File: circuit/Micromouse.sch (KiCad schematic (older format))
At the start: 34 parts, among them J1 DBG_CN, J2 ICM-20602_1-4pin, J3 TEST_1P, J4 ICM-20602_5-8pin, J5 TEST_1P, J6 Conn_01x04, Q2 IRLML6344, SW2 SW_Push, SW3 SW_Push, SW4 SW_Push, U3 STM32F405RGTx

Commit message: Kicadのpcbnew映らないくてキレそう
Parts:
- D2, D3, D4, D5: footprint (none) -> LEDs:LED_0603
- J1: footprint (none) -> Socket_Strips:Socket_Strip_Straight_1x03_Pitch2.54mm
- J2, J4, J6: footprint (none) -> Socket_Strips:Socket_Strip_Straight_1x04_Pitch2.54mm
- R10, R5, R6, R9: footprint (none) -> Resistors_SMD:R_0603
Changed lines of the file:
@@
 F 0 "J4" H 5750 8650 50  0000 C CNN
 F 1 "ICM-20602_5-8pin" V 5850 8850 50  0000 C CNN
-F 2 "" H 5750 8950 50  0001 C CNN
+F 2 "Socket_Strips:Socket_Strip_Straight_1x04_Pitch2.54mm" H 5750 8950 50  0001 C CNN
 F 3 "~" H 5750 8950 50  0001 C CNN
 	1    5750 8950
@@
 F 0 "J6" H 12530 1742 50  0000 L CNN
 F 1 "Conn_01x04" H 12530 1651 50  0000 L CNN
-F 2 "" H 12450 1750 50  0001 C CNN
+F 2 "Socket_Strips:Socket_Strip_Straight_1x04_Pitch2.54mm" H 12450 1750 50  0001 C CNN
 F 3 "~" H 12450 1750 50  0001 C CNN
 	1    12450 1750
@@
 F 0 "R10" H 3670 10146 50  0000 L CNN
 F 1 "10k" H 3670 10055 50  0000 L CNN
-F 2 "" V 3530 10100 50  0001 C CNN
+F 2 "Resistors_SMD:R_0603" V 3530 10100 50  0001 C CNN
 F 3 "" H 3600 10100 50  0001 C CNN
 	1    3600 10100
@@
 F 0 "D5" V 3639 9532 50  0000 R CNN
 F 1 "DBG_LED2" V 3548 9532 50  0000 R CNN
-F 2 "" H 3600 9650 50  0001 C CNN
+F 2 "LEDs:LED_0603" H 3600 9650 50  0001 C CNN
 F 3 "" H 3600 9650 50  0001 C CNN
 	1    3600 9650
@@
 F 0 "J1" H 4618 9525 50  0000 C CNN
 F 1 "DBG_CN" H 4618 9616 50  0000 C CNN
-F 2 "" H 4700 9850 50  0001 C CNN
+F 2 "Socket_Strips:Socket_Strip_Straight_1x03_Pitch2.54mm" H 4700 9850 50  0001 C CNN
 F 3 "~" H 4700 9850 50  0001 C CNN
 	1    4700 9850
@@
 F 0 "R9" H 2970 10146 50  0000 L CNN
 F 1 "10k" H 2970 10055 50  0000 L CNN
-F 2 "" V 2830 10100 50  0001 C CNN
+F 2 "Resistors_SMD:R_0603" V 2830 10100 50  0001 C CNN
 F 3 "" H 2900 10100 50  0001 C CNN
 	1    2900 10100
@@
 F 0 "R6" H 2220 10146 50  0000 L CNN
 F 1 "10k" H 2220 10055 50  0000 L CNN
-F 2 "" V 2080 10100 50  0001 C CNN
+F 2 "Resistors_SMD:R_0603" V 2080 10100 50  0001 C CNN
 F 3 "" H 2150 10100 50  0001 C CNN
 	1    2150 10100
@@
 F 0 "R5" H 1470 10146 50  0000 L CNN
 F 1 "10k" H 1470 10055 50  0000 L CNN
-F 2 "" V 1330 10100 50  0001 C CNN
+F 2 "Resistors_SMD:R_0603" V 1330 10100 50  0001 C CNN
 F 3 "" H 1400 10100 50  0001 C CNN
 	1    1400 10100
@@
 F 0 "D4" V 2939 9532 50  0000 R CNN
 F 1 "DBG_LED1" V 2848 9532 50  0000 R CNN
-F 2 "" H 2900 9650 50  0001 C CNN
+F 2 "LEDs:LED_0603" H 2900 9650 50  0001 C CNN
 F 3 "" H 2900 9650 50  0001 C CNN
 	1    2900 9650
@@
 F 0 "D3" V 2189 9532 50  0000 R CNN
 F 1 "DBG_LED0" V 2098 9532 50  0000 R CNN
-F 2 "" H 2150 9650 50  0001 C CNN
+F 2 "LEDs:LED_0603" H 2150 9650 50  0001 C CNN
 F 3 "" H 2150 9650 50  0001 C CNN
 	1    2150 9650
@@
 F 0 "D2" V 1439 9533 50  0000 R CNN
 F 1 "TICK_LED" V 1348 9533 50  0000 R CNN
-F 2 "" H 1400 9650 50  0001 C CNN
+F 2 "LEDs:LED_0603" H 1400 9650 50  0001 C CNN
 F 3 "" H 1400 9650 50  0001 C CNN
 	1    1400 9650
@@
 F 0 "J2" H 5200 9050 50  0000 C CNN
 F 1 "ICM-20602_1-4pin" V 5300 8850 50  0000 C CNN
-F 2 "" H 5200 8850 50  0001 C CNN
+F 2 "Socket_Strips:Socket_Strip_Straight_1x04_Pitch2.54mm" H 5200 8850 50  0001 C CNN
 F 3 "~" H 5200 8850 50  0001 C CNN
 	1    5200 8850

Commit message: スーパーエンジニアの登竜門たる文彦は当然スーパーエンジニア
あってぃ許さない
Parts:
- C10, C11, C12, C13, C14, C15, C23, C5, C6, C7, C8, C9: footprint Capacitors_SMD:C_0603 -> Capacitor_SMD:C_0603_1608Metric
- D2, D3, D4, D5: footprint LEDs:LED_0603 -> LED_SMD:LED_0603_1608Metric
- J1: footprint Socket_Strips:Socket_Strip_Straight_1x03_Pitch2.54mm -> Connector_PinSocket_2.54mm:PinSocket_1x03_P2.54mm_Vertical
- J2, J4, J6: footprint Socket_Strips:Socket_Strip_Straight_1x04_Pitch2.54mm -> Connector_PinSocket_2.54mm:PinSocket_1x04_P2.54mm_Vertical
- J3, J5: footprint Measurement_Points:Measurement_Point_Round-SMD-Pad_Small -> TestPoint:TestPoint_Pad_D1.0mm
- LS1: symbol Audio:CSS-0575A-SMT -> Micromouse-rescue:CSS-0575A-SMT-Audio
- Q2: footprint TO_SOT_Packages_SMD:SOT-23 -> Package_TO_SOT_SMD:SOT-23
- R10, R5, R6, R7, R8, R9: footprint Resistors_SMD:R_0603 -> Resistor_SMD:R_0603_1608Metric
- U3: footprint LQFP64 -> Package_QFP:LQFP-64_10x10mm_P0.5mm
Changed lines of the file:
@@
 F 0 "J4" H 5750 8650 50  0000 C CNN
 F 1 "ICM-20602_5-8pin" V 5850 8850 50  0000 C CNN
-F 2 "Socket_Strips:Socket_Strip_Straight_1x04_Pitch2.54mm" H 5750 8950 50  0001 C CNN
+F 2 "Connector_PinSocket_2.54mm:PinSocket_1x04_P2.54mm_Vertical" H 5750 8950 50  0001 C CNN
 F 3 "~" H 5750 8950 50  0001 C CNN
 	1    5750 8950
@@
 F 0 "C23" H 9065 4546 50  0000 L CNN
 F 1 "2.2u" H 9065 4455 50  0000 L CNN
-F 2 "Capacitors_SMD:C_0603" H 8988 4350 50  0001 C CNN
+F 2 "Capacitor_SMD:C_0603_1608Metric" H 8988 4350 50  0001 C CNN
 F 3 "" H 8950 4500 50  0001 C CNN
 	1    8950 4500
@@
 F 0 "C8" H 9015 8796 50  0000 L CNN
 F 1 "0.1u" H 9015 8705 50  0000 L CNN
-F 2 "Capacitors_SMD:C_0603" H 8938 8600 50  0001 C CNN
+F 2 "Capacitor_SMD:C_0603_1608Metric" H 8938 8600 50  0001 C CNN
 F 3 "" H 8900 8750 50  0001 C CNN
 	1    8900 8750
@@
 F 0 "C5" H 7865 8796 50  0000 L CNN
 F 1 "0.1u" H 7865 8705 50  0000 L CNN
-F 2 "Capacitors_SMD:C_0603" H 7788 8600 50  0001 C CNN
+F 2 "Capacitor_SMD:C_0603_1608Metric" H 7788 8600 50  0001 C CNN
 F 3 "" H 7750 8750 50  0001 C CNN
 	1    7750 8750
@@
 F 0 "J3" H 5750 10100 50  0000 L CNN
 F 1 "TEST_1P" H 5650 10000 50  0000 L CNN
-F 2 "Measurement_Points:Measurement_Point_Round-SMD-Pad_Small" H 6000 9800 50  0001 C CNN
+F 2 "TestPoint:TestPoint_Pad_D1.0mm" H 6000 9800 50  0001 C CNN
 F 3 "" H 6000 9800 50  0001 C CNN
 	1    5800 9800
@@
 F 0 "J5" H 6100 10100 50  0000 L CNN
 F 1 "TEST_1P" H 6000 10000 50  0000 L CNN
-F 2 "Measurement_Points:Measurement_Point_Round-SMD-Pad_Small" H 6350 9800 50  0001 C CNN
+F 2 "TestPoint:TestPoint_Pad_D1.0mm" H 6350 9800 50  0001 C CNN
 F 3 "" H 6350 9800 50  0001 C CNN
 	1    6150 9800
@@
 F 0 "J6" H 12530 1742 50  0000 L CNN
 F 1 "Conn_01x04" H 12530 1651 50  0000 L CNN
-F 2 "Socket_Strips:Socket_Strip_Straight_1x04_Pitch2.54mm" H 12450 1750 50  0001 C CNN
+F 2 "Connector_PinSocket_2.54mm:PinSocket_1x04_P2.54mm_Vertical" H 12450 1750 50  0001 C CNN
 F 3 "~" H 12450 1750 50  0001 C CNN
 	1    12450 1750
@@
 F 0 "R10" H 3670 10146 50  0000 L CNN
 F 1 "10k" H 3670 10055 50  0000 L CNN
-F 2 "Resistors_SMD:R_0603" V 3530 10100 50  0001 C CNN
+F 2 "Resistor_SMD:R_0603_1608Metric" V 3530 10100 50  0001 C CNN
 F 3 "" H 3600 10100 50  0001 C CNN
 	1    3600 10100
@@
 F 0 "D5" V 3639 9532 50  0000 R CNN
 F 1 "DBG_LED2" V 3548 9532 50  0000 R CNN
-F 2 "LEDs:LED_0603" H 3600 9650 50  0001 C CNN
+F 2 "LED_SMD:LED_0603_1608Metric" H 3600 9650 50  0001 C CNN
 F 3 "" H 3600 9650 50  0001 C CNN
 	1    3600 9650
@@
 $EndComp
 $Comp
-L Audio:CSS-0575A-SMT LS1
+L Micromouse-rescue:CSS-0575A-SMT-Audio LS1
 U 1 1 5FB2CA92
 P 2650 6950
@@
 F 0 "R7" V 2207 7450 50  0000 C CNN
 F 1 "10" V 2116 7450 50  0000 C CNN
-F 2 "Resistors_SMD:R_0603" V 1930 7450 50  0001 C CNN
+F 2 "Resistor_SMD:R_0603_1608Metric" V 1930 7450 50  0001 C CNN
 F 3 "" H 2000 7450 50  0001 C CNN
 	1    2000 7450
@@
 F 0 "R8" H 2320 7696 50  0000 L CNN
 F 1 "10k" H 2320 7605 50  0000 L CNN
-F 2 "Resistors_SMD:R_0603" V 2180 7650 50  0001 C CNN
+F 2 "Resistor_SMD:R_0603_1608Metric" V 2180 7650 50  0001 C CNN
 F 3 "" H 2250 7650 50  0001 C CNN
 	1    2250 7650
@@
 F 0 "Q2" H 2756 7496 50  0000 L CNN
 F 1 "IRLML6344" H 2756 7405 50  0000 L CNN
-F 2 "TO_SOT_Packages_SMD:SOT-23" H 2750 7550 50  0001 C CNN
+F 2 "Package_TO_SOT_SMD:SOT-23" H 2750 7550 50  0001 C CNN
 F 3 "https://akizukidenshi.com/download/ds/ir/irlml6344pbf.pdf" H 2550 7450 50  0001 C CNN
 	1    2550 7450
@@
 F 0 "J1" H 4618 9525 50  0000 C CNN
 F 1 "DBG_CN" H 4618 9616 50  0000 C CNN
-F 2 "Socket_Strips:Socket_Strip_Straight_1x03_Pitch2.54mm" H 4700 9850 50  0001 C CNN
+F 2 "Connector_PinSocket_2.54mm:PinSocket_1x03_P2.54mm_Vertical" H 4700 9850 50  0001 C CNN
 F 3 "~" H 4700 9850 50  0001 C CNN
 	1    4700 9850
@@
 F 0 "R9" H 2970 10146 50  0000 L CNN
 F 1 "10k" H 2970 10055 50  0000 L CNN
-F 2 "Resistors_SMD:R_0603" V 2830 10100 50  0001 C CNN
+F 2 "Resistor_SMD:R_0603_1608Metric" V 2830 10100 50  0001 C CNN
 F 3 "" H 2900 10100 50  0001 C CNN
 	1    2900 10100
@@
 F 0 "R6" H 2220 10146 50  0000 L CNN
 F 1 "10k" H 2220 10055 50  0000 L CNN
-F 2 "Resistors_SMD:R_0603" V 2080 10100 50  0001 C CNN
+F 2 "Resistor_SMD:R_0603_1608Metric" V 2080 10100 50  0001 C CNN
 F 3 "" H 2150 10100 50  0001 C CNN
 	1    2150 10100
@@
 F 0 "R5" H 1470 10146 50  0000 L CNN
 F 1 "10k" H 1470 10055 50  0000 L CNN
-F 2 "Resistors_SMD:R_0603" V 1330 10100 50  0001 C CNN
+F 2 "Resistor_SMD:R_0603_1608Metric" V 1330 10100 50  0001 C CNN
 F 3 "" H 1400 10100 50  0001 C CNN
 	1    1400 10100
@@
 F 0 "D4" V 2939 9532 50  0000 R CNN
 F 1 "DBG_LED1" V 2848 9532 50  0000 R CNN
-F 2 "LEDs:LED_0603" H 2900 9650 50  0001 C CNN
+F 2 "LED_SMD:LED_0603_1608Metric" H 2900 9650 50  0001 C CNN
 F 3 "" H 2900 9650 50  0001 C CNN
 	1    2900 9650
@@
 F 0 "D3" V 2189 9532 50  0000 R CNN
 F 1 "DBG_LED0" V 2098 9532 50  0000 R CNN
-F 2 "LEDs:LED_0603" H 2150 9650 50  0001 C CNN
+F 2 "LED_SMD:LED_0603_1608Metric" H 2150 9650 50  0001 C CNN
 F 3 "" H 2150 9650 50  0001 C CNN
 	1    2150 9650
@@
 F 0 "D2" V 1439 9533 50  0000 R CNN
 F 1 "TICK_LED" V 1348 9533 50  0000 R CNN
-F 2 "LEDs:LED_0603" H 1400 9650 50  0001 C CNN
+F 2 "LED_SMD:LED_0603_1608Metric" H 1400 9650 50  0001 C CNN
 F 3 "" H 1400 9650 50  0001 C CNN
 	1    1400 9650
@@
 F 0 "C7" V 8300 3500 50  0000 C CNN
 F 1 "0.1u" V 8400 3500 50  0000 C CNN
-F 2 "Capacitors_SMD:C_0603" H 8188 3350 50  0001 C CNN
+F 2 "Capacitor_SMD:C_0603_1608Metric" H 8188 3350 50  0001 C CNN
 F 3 "" H 8150 3500 50  0001 C CNN
 	1    8150 3500
 	0    1    1    0
-$EndComp
-$Comp
-L MCU_ST_STM32F4:STM32F405RGTx U3
-U 1 1 5F9C187D
-P 10150 5400
-F 0 "U3" H 9850 3400 50  0000 C CNN
-F 1 "STM32F405RGTx" H 10750 3400 50  0000 C CNN
-F 2 "LQFP64" H 14350 7275 50  0001 R TNN
-F 3 "http://www.st.com/st-web-ui/static/active/en/resource/technical/document/datasheet/DM00037051.pdf" H 10150 5400 50  0001 C CNN
-	1    10150 5400
-	1    0    0    -1
 $EndComp
 $Comp
@@
 F 0 "C15" V 10548 3100 50  0000 C CNN
 F 1 "1u" V 10639 3100 50  0000 C CNN
-F 2 "Capacitors_SMD:C_0603" H 10838 2950 50  0001 C CNN
+F 2 "Capacitor_SMD:C_0603_1608Metric" H 10838 2950 50  0001 C CNN
 F 3 "" H 10800 3100 50  0001 C CNN
 	1    10800 3100
@@
 F 0 "C14" V 10548 2700 50  0000 C CNN
 F 1 "0.1u" V 10639 2700 50  0000 C CNN
-F 2 "Capacitors_SMD:C_0603" H 10838 2550 50  0001 C CNN
+F 2 "Capacitor_SMD:C_0603_1608Metric" H 10838 2550 50  0001 C CNN
 F 3 "" H 10800 2700 50  0001 C CNN
 	1    10800 2700
@@
 F 0 "C9" V 9398 1350 50  0000 C CNN
 F 1 "4.7u" V 9489 1350 50  0000 C CNN
-F 2 "Capacitors_SMD:C_0603" H 9688 1200 50  0001 C CNN
+F 2 "Capacitor_SMD:C_0603_1608Metric" H 9688 1200 50  0001 C CNN
 F 3 "" H 9650 1350 50  0001 C CNN
 	1    9650 1350
@@
 F 0 "C13" V 9398 2950 50  0000 C CNN
 F 1 "0.1u" V 9489 2950 50  0000 C CNN
-F 2 "Capacitors_SMD:C_0603" H 9688 2800 50  0001 C CNN
+F 2 "Capacitor_SMD:C_0603_1608Metric" H 9688 2800 50  0001 C CNN
 F 3 "" H 9650 2950 50  0001 C CNN
 	1    9650 2950
@@
 F 0 "C12" V 9398 2550 50  0000 C CNN
 F 1 "0.1u" V 9489 2550 50  0000 C CNN
-F 2 "Capacitors_SMD:C_0603" H 9688 2400 50  0001 C CNN
+F 2 "Capacitor_SMD:C_0603_1608Metric" H 9688 2400 50  0001 C CNN
 F 3 "" H 9650 2550 50  0001 C CNN
 	1    9650 2550
@@
 F 0 "C11" V 9398 2150 50  0000 C CNN
 F 1 "0.1u" V 9489 2150 50  0000 C CNN
-F 2 "Capacitors_SMD:C_0603" H 9688 2000 50  0001 C CNN
+F 2 "Capacitor_SMD:C_0603_1608Metric" H 9688 2000 50  0001 C CNN
 F 3 "" H 9650 2150 50  0001 C CNN
 	1    9650 2150
@@
 F 0 "C6" H 8615 4546 50  0000 L CNN
 F 1 "2.2u" H 8615 4455 50  0000 L CNN
-F 2 "Capacitors_SMD:C_0603" H 8538 4350 50  0001 C CNN
+F 2 "Capacitor_SMD:C_0603_1608Metric" H 8538 4350 50  0001 C CNN
 F 3 "" H 8500 4500 50  0001 C CNN
 	1    8500 4500
@@
 F 0 "C10" V 9398 1750 50  0000 C CNN
 F 1 "0.1u" V 9489 1750 50  0000 C CNN
-F 2 "Capacitors_SMD:C_0603" H 9688 1600 50  0001 C CNN
+F 2 "Capacitor_SMD:C_0603_1608Metric" H 9688 1600 50  0001 C CNN
 F 3 "" H 9650 1750 50  0001 C CNN
 	1    9650 1750
@@
 F 0 "J2" H 5200 9050 50  0000 C CNN
 F 1 "ICM-20602_1-4pin" V 5300 8850 50  0000 C CNN
-F 2 "Socket_Strips:Socket_Strip_Straight_1x04_Pitch2.54mm" H 5200 8850 50  0001 C CNN
+F 2 "Connector_PinSocket_2.54mm:PinSocket_1x04_P2.54mm_Vertical" H 5200 8850 50  0001 C CNN
 F 3 "~" H 5200 8850 50  0001 C CNN
 	1    5200 8850
@@
 Wire Wire Line
 	4900 9950 5000 9950
+$Comp
+L MCU_ST_STM32F4:STM32F405RGTx U3
+U 1 1 5FB0A9CA
+P 10150 5400
+F 0 "U3" H 10150 3511 50  0000 C CNN
+F 1 "STM32F405RGTx" H 10150 3420 50  0000 C CNN
+F 2 "Package_QFP:LQFP-64_10x10mm_P0.5mm" H 9550 3700 50  0001 R CNN
+F 3 "http://www.st.com/st-web-ui/static/active/en/resource/technical/document/datasheet/DM00037051.pdf" H 10150 5400 50  0001 C CNN
+	1    10150 5400
+	1    0    0    -1
+$EndComp
 $EndSCHEMATC

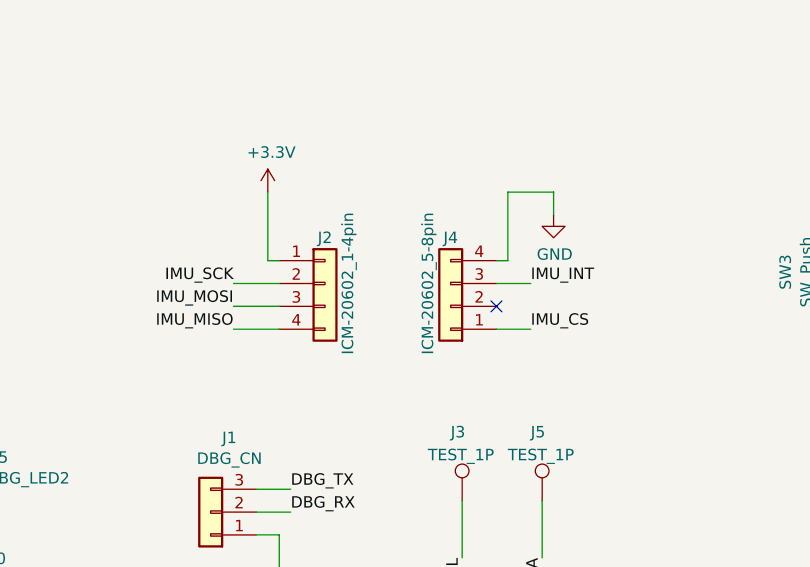
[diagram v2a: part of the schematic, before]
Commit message: AW何も分からん
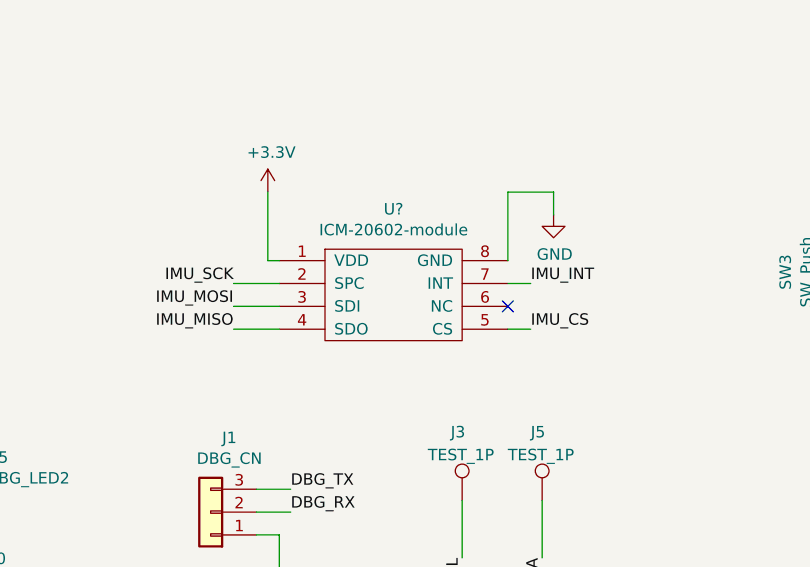
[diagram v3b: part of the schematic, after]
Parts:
- removed J2: ICM-20602_1-4pin, Connector_PinSocket_2.54mm:PinSocket_1x04_P2.54mm_Vertical, symbol Connector_Generic:Conn_01x04
- removed J4: ICM-20602_5-8pin, Connector_PinSocket_2.54mm:PinSocket_1x04_P2.54mm_Vertical, symbol Connector_Generic:Conn_01x04
- added U?: ICM-20602-module, Original:ICM-20602, symbol Sensor_Motion:ICM-20602-module
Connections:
- net +3V3: now also U?.1 (VDD)
- net GND: now also U?.8 (GND)
- net IMU_CS: now also U?.5 (CS)
- net IMU_INT: now also U?.7 (INT)
- net IMU_MISO: now also U?.4 (SDO)
- net IMU_MOSI: now also U?.3 (SDI)
- net IMU_SCK: now also U?.2 (SPC)
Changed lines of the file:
@@
 	6200 8550 6200 8450
 Wire Wire Line
-	5950 8750 6000 8750
-Wire Wire Line
 	6000 8750 6000 8450
-NoConn ~ 5950 8950
-Wire Wire Line
-	5950 8850 6100 8850
-Wire Wire Line
-	5950 9050 6100 9050
 Wire Wire Line
 	1400 10250 1400 10350
@@
 	9450 3900 9450 4000
 $Comp
-L Connector_Generic:Conn_01x04 J4
-U 1 1 5F9E478F
-P 5750 8950
-F 0 "J4" H 5750 8650 50  0000 C CNN
-F 1 "ICM-20602_5-8pin" V 5850 8850 50  0000 C CNN
-F 2 "Connector_PinSocket_2.54mm:PinSocket_1x04_P2.54mm_Vertical" H 5750 8950 50  0001 C CNN
-F 3 "~" H 5750 8950 50  0001 C CNN
-	1    5750 8950
-	-1   0    0    1
-$EndComp
-$Comp
 L Device:C C23
 U 1 1 5FA4F16F
@@
 Wire Wire Line
 	4800 8850 5000 8850
-$Comp
-L Connector_Generic:Conn_01x04 J2
-U 1 1 5F9DF759
-P 5200 8850
-F 0 "J2" H 5200 9050 50  0000 C CNN
-F 1 "ICM-20602_1-4pin" V 5300 8850 50  0000 C CNN
-F 2 "Connector_PinSocket_2.54mm:PinSocket_1x04_P2.54mm_Vertical" H 5200 8850 50  0001 C CNN
-F 3 "~" H 5200 8850 50  0001 C CNN
-	1    5200 8850
-	1    0    0    -1
-$EndComp
 Wire Wire Line
 	4900 9750 5050 9750
@@
 	1    0    0    -1
 $EndComp
+$Comp
+L Sensor_Motion:ICM-20602-module U?
+U 1 1 5FBFC8AB
+P 5500 8900
+F 0 "U?" H 5500 9275 50  0000 C CNN
+F 1 "ICM-20602-module" H 5500 9184 50  0000 C CNN
+F 2 "Original:ICM-20602" H 5500 8900 50  0001 C CNN
+F 3 "" H 5500 8900 50  0001 C CNN
+	1    5500 8900
+	1    0    0    -1
+$EndComp
+Wire Wire Line
+	6000 9050 6100 9050
+Wire Wire Line
+	6000 8850 6100 8850
+NoConn ~ 6000 8950
 $EndSCHEMATC
